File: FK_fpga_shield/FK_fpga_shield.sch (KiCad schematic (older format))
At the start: 172 parts, among them J0 USB_B_Mini, J1 molex-51382-0400-microclasp, J10 molex-51382-0400-microclasp, J11 molex-51382-0400-microclasp, J12 molex-51382-0400-microclasp, J13 molex-51382-0400-microclasp, J14 molex-51382-0400-microclasp, J15 molex-51382-0400-microclasp, J16 molex-51382-0400-microclasp, J17 molex-51382-0400-microclasp, J18 molex-51382-0400-microclasp, J19 molex-51382-0400-microclasp, J2 molex-51382-0400-microclasp, J20 molex-51382-0400-microclasp, J21 molex-51382-0400-microclasp, J22 molex-51382-0400-microclasp, J23 molex-51382-0400-microclasp, J24 molex-51382-0400-microclasp, J25 molex-51382-0400-microclasp, J26 molex-51382-0400-microclasp, J27 molex-51382-0400-microclasp, J28 molex-51382-0400-microclasp, J29 molex-51382-0400-microclasp, J3 molex-51382-0400-microclasp, J30 molex-51382-0400-microclasp, J31 molex-51382-0400-microclasp, J32 molex-51382-0400-microclasp, J33 molex-51382-0400-microclasp, J34 molex-51382-0400-microclasp, J35 molex-51382-0400-microclasp, J36 Barrel_Jack_MountingPin, J37 Conn_02x04_Top_Bottom, J4 molex-51382-0400-microclasp, J5 molex-51382-0400-microclasp, J6 molex-51382-0400-microclasp, J7 molex-51382-0400-microclasp, J8 molex-51382-0400-microclasp, J9 molex-51382-0400-microclasp, U1 FT232RL, U2 nvt2010pw, U3 nvt2010pw, U4 nvt2010pw, U5 nvt2010pw, U6 nvt2010pw, U7 nvt2010pw, U8 nvt2010pw, Y1 DNP_(12MHz)

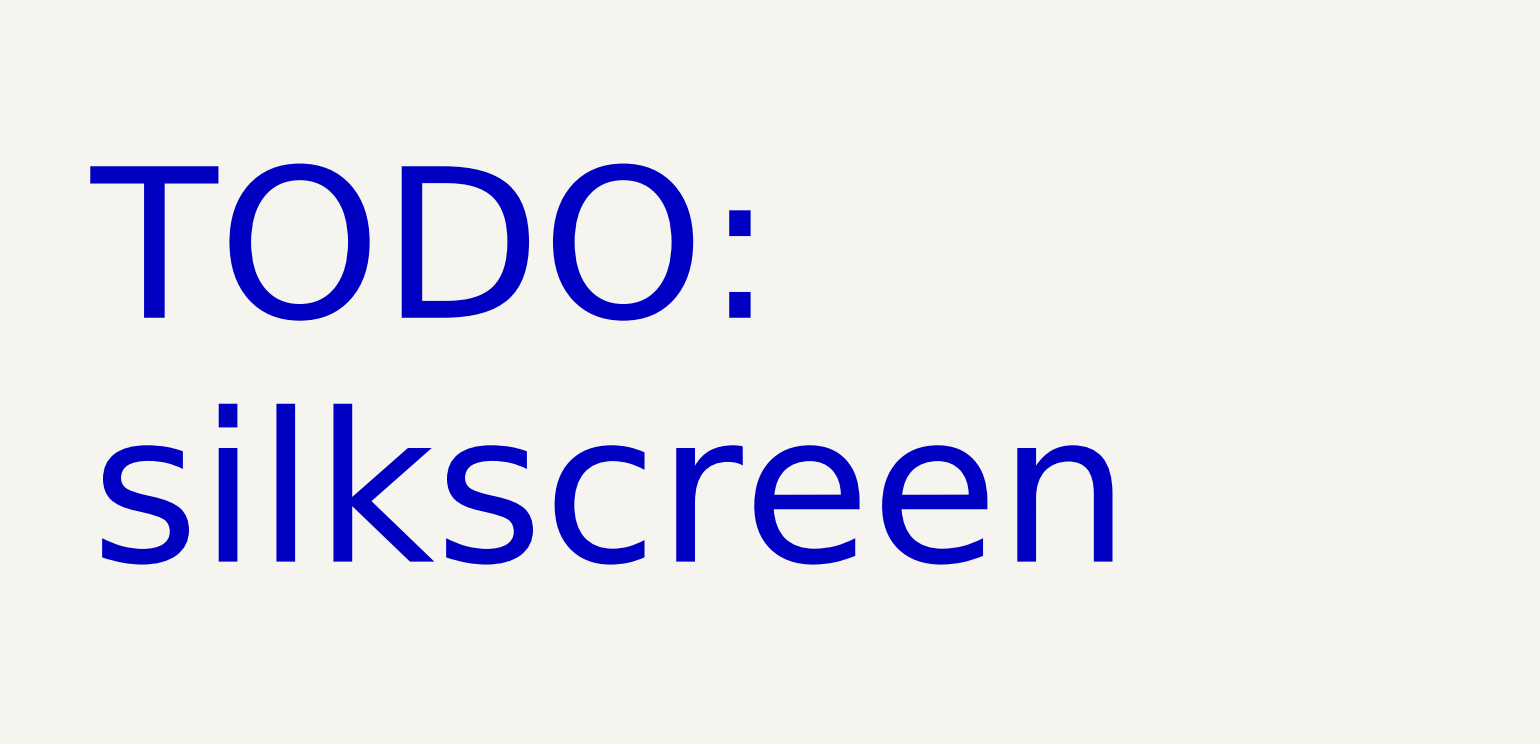
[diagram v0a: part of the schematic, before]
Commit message: gerbers etc
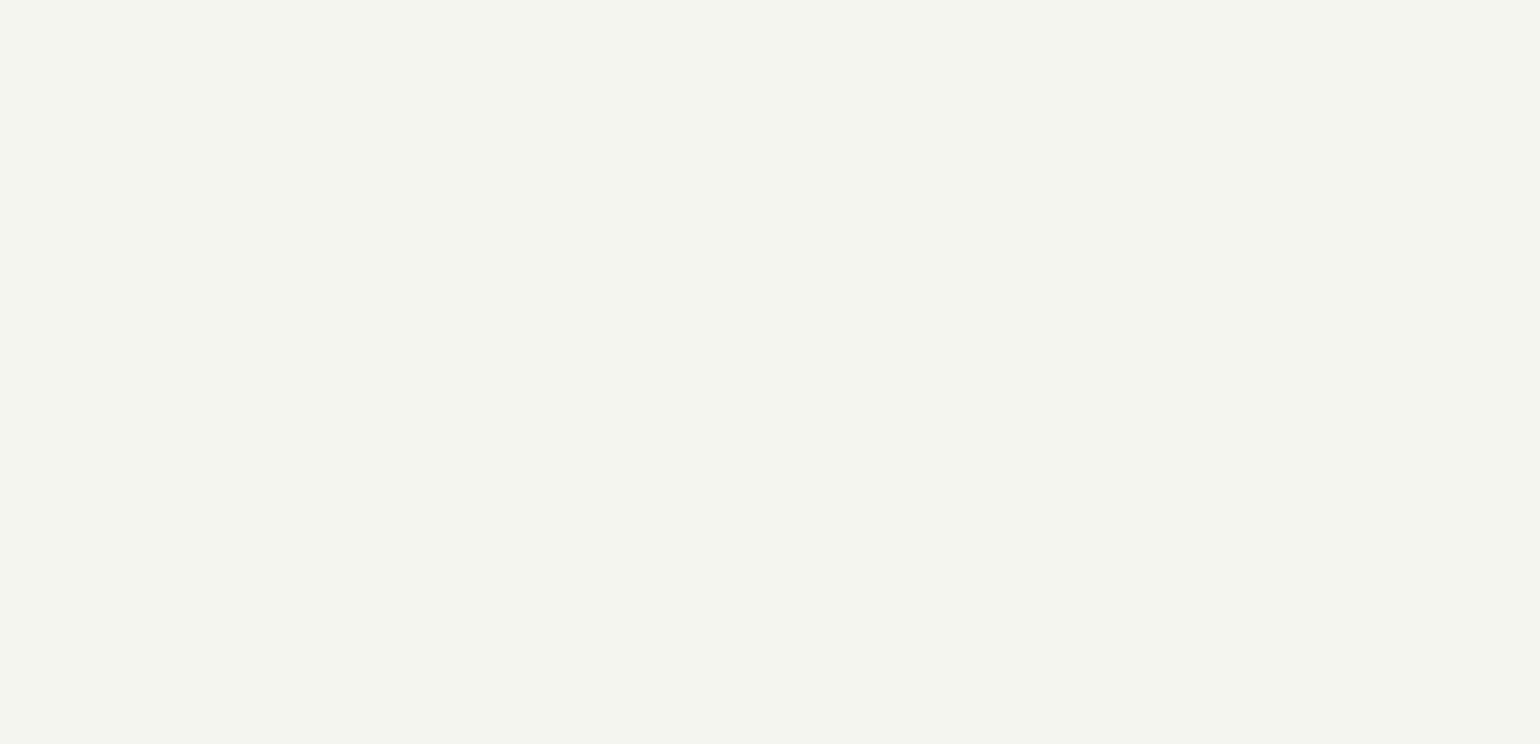
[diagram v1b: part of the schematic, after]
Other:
- note removed: "TODO:\nsilkscreen"
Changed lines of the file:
@@
 Text Label 14250 2950 0    50   ~ 0
 3V3
-Text Notes 16650 7750 0    1181 ~ 0
-TODO:\nsilkscreen
 $Comp
 L FK_fpga_shield_custom_symbols:BNX016-01 FL1
